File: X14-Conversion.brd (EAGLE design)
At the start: 50.8 x 62.9 mm, 25 parts, among them U1 BUCK,LM2678S-ADJ

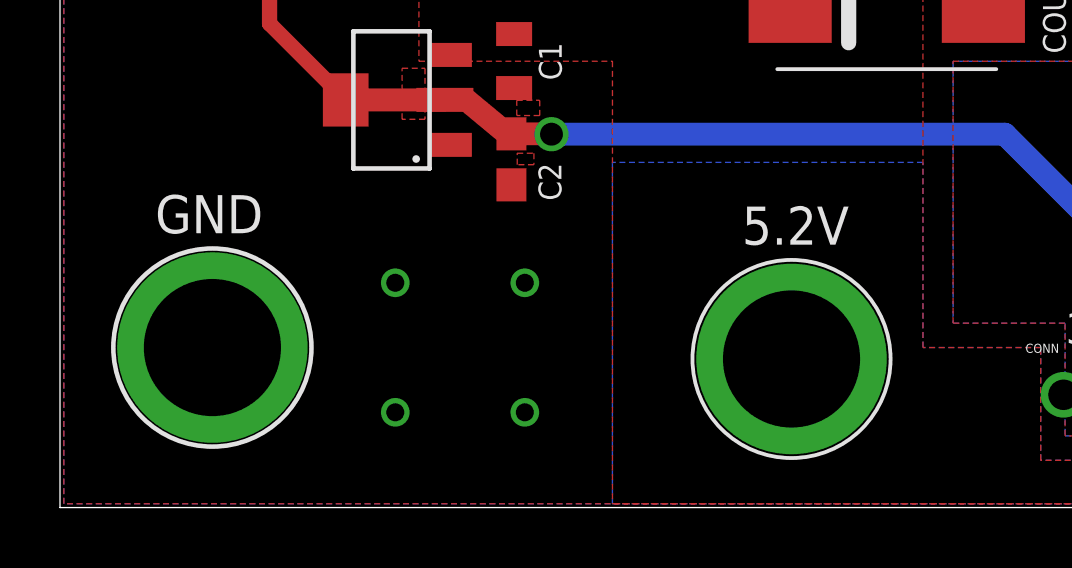
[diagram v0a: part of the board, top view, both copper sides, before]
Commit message: Update X14-Conversion.brd
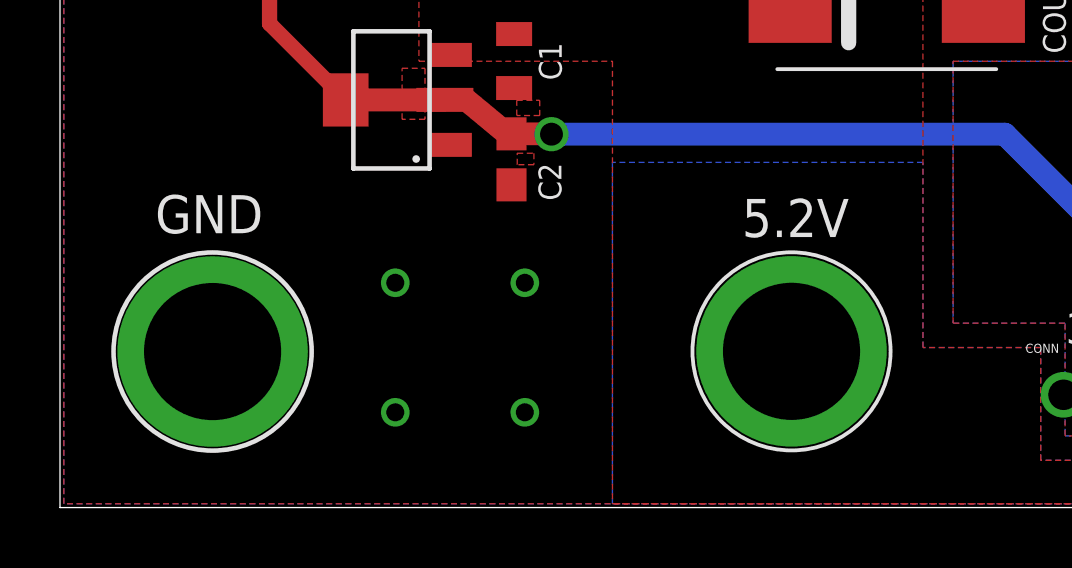
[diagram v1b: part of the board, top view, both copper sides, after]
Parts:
- moved U$3 0.25 mm to (24.4, 10.9)
- moved U$6 0.13 mm to (5.09, 10.9)
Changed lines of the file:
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@@
 <wire x1="35.56" y1="53.34" x2="50.8" y2="53.34" width="0" layer="20"/>
 <text x="44.45" y="38.1" size="1.27" layer="21">12V</text>
-<text x="22.733" y="14.478" size="1.27" layer="21">5.2V</text>
+<text x="22.733" y="14.732" size="1.27" layer="21">5.2V</text>
 <text x="44.069" y="20.32" size="1.27" layer="21">3.3V</text>
 <text x="43.942" y="26.035" size="1.27" layer="21">GND</text>
@@
 </element>
 <element name="U$2" library="testpoints" package="3.3V_TESTPOINT" value="3.3V_TESTPOINT" x="45.974" y="16.51" smashed="yes"/>
-<element name="U$3" library="testpoints" package="5.2V_TESTPOINT" value="5.2V_TESTPOINT" x="24.384" y="10.668" smashed="yes"/>
+<element name="U$3" library="testpoints" package="5.2V_TESTPOINT" value="5.2V_TESTPOINT" x="24.384" y="10.922" smashed="yes"/>
 <element name="U$4" library="testpoints" package="12V_TESTPOINT" value="12V_TESTPOINT" x="45.974" y="42.672" smashed="yes"/>
 <element name="U$5" library="testpoints" package="GND_TESTPOINT" value="GND_TESTPOINT" x="30.607" y="63.627" smashed="yes"/>
-<element name="U$6" library="testpoints" package="GND_TESTPOINT" value="GND_TESTPOINT" x="5.08" y="11.049" smashed="yes"/>
+<element name="U$6" library="testpoints" package="GND_TESTPOINT" value="GND_TESTPOINT" x="5.08635" y="10.91565" smashed="yes"/>
 <element name="U$7" library="testpoints" package="GND_TESTPOINT" value="GND_TESTPOINT" x="45.974" y="30.988" smashed="yes"/>
 <element name="RFB2" library="SparkFun-Resistors" library_urn="urn:adsk.eagle:library:532" package="0603" package3d_urn="urn:adsk.eagle:package:39650/1" value="3.32kΩ" x="27.305" y="39.37" smashed="yes" rot="R270">
